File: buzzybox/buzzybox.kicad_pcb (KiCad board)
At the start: 2 copper layers, 116.8 x 71.1 mm, 67 parts, among them J1 AudioJack2, J2 Barrel_Jack, Q1 Q_NPN_EBC, Q10 Q_NPN_EBC, Q2 Q_NPN_EBC, Q3 Q_NPN_EBC, Q4 Q_NPN_EBC, Q5 Q_NPN_EBC, Q6 Q_NPN_EBC, Q7 Q_NPN_EBC, Q8 Q_NPN_EBC, Q9 Q_NPN_EBC

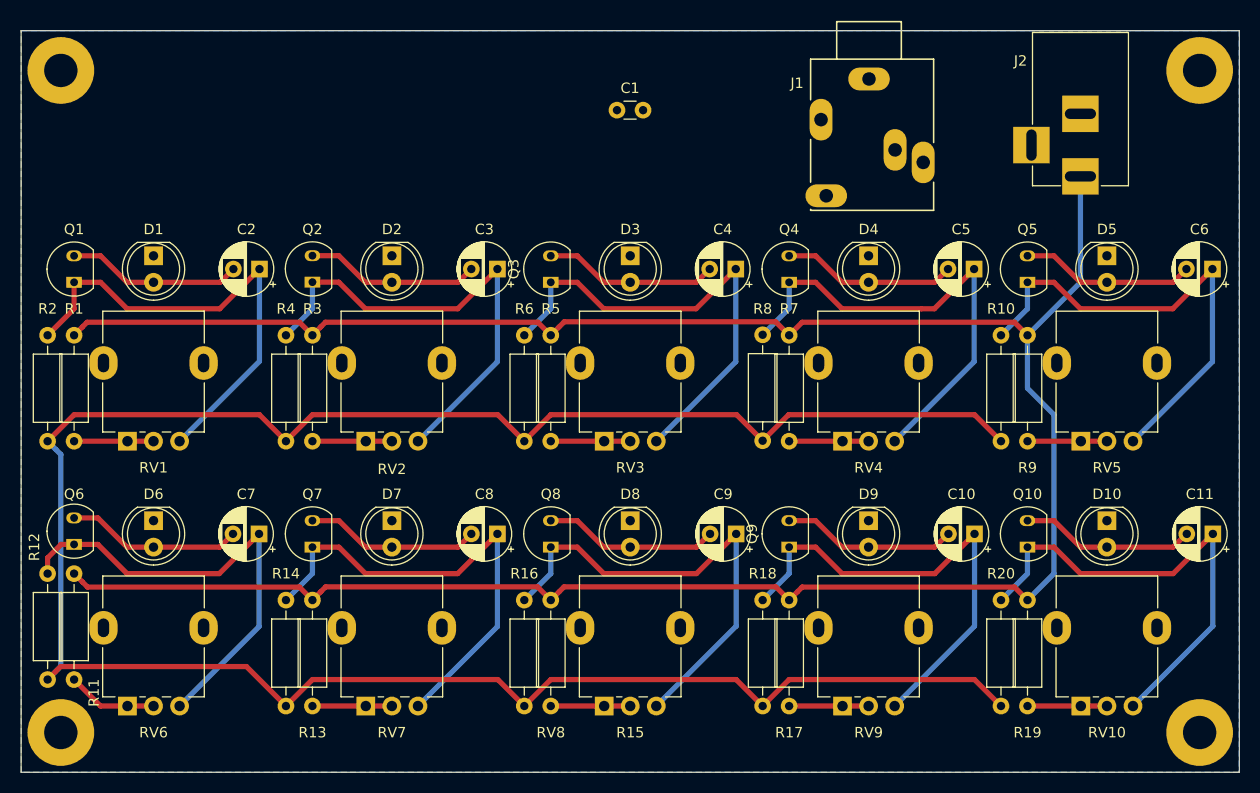
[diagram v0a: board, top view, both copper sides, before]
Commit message: complete mini layout
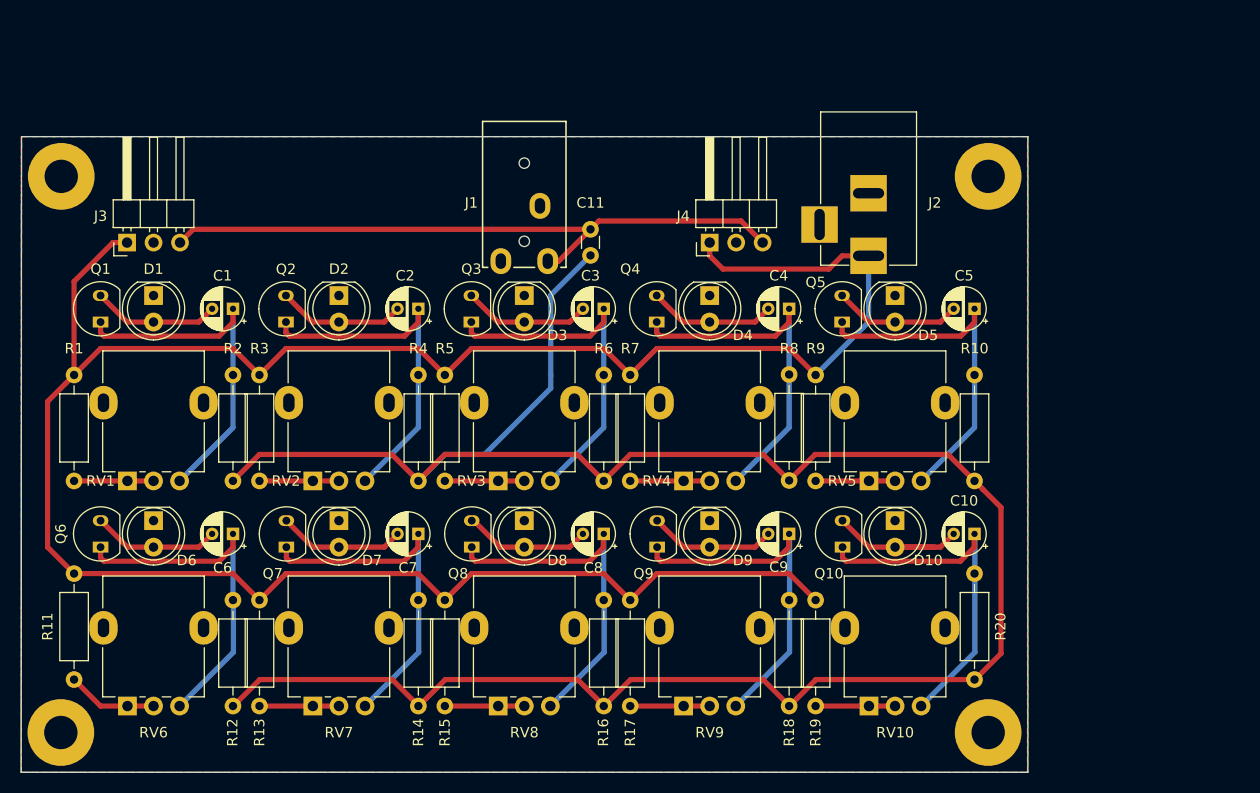
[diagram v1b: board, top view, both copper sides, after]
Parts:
- removed the C11 at (177.8, 87.6)
- added C1: CP1, Capacitor_THT:CP_Radial_D4.0mm_P2.00mm, F.Cu at (83.8, 66.0)
- added J3: Conn_01x03, Connector_PinHeader_2.54mm:PinHeader_1x03_P2.54mm_Horizontal, F.Cu at (73.7, 59.7)
- added J4: Conn_01x03, Connector_PinHeader_2.54mm:PinHeader_1x03_P2.54mm_Horizontal, F.Cu at (129.5, 59.7)
- C10, C2, C3, C4, C5, C6, C7, C8, C9: value C -> CP1; footprint Capacitor_THT:CP_Radial_D5.0mm_P2.50mm -> Capacitor_THT:CP_Radial_D4.0mm_P2.00mm
- J1: value AudioJack2 -> AudioJack3; footprint Connectors:Stereo_Jack_3.5mm_Switch_Ledino_KB3SPRS -> buzzybox:STX-3000
- Q1, Q10, Q2, Q3, Q4, Q5, Q6, Q7, Q8, Q9: value Q_NPN_EBC -> NPN
- moved C6 97.3 mm to (83.8, 87.6)
- moved J1 28.8 mm to (111.8, 52.1), turned to 0 degrees
- moved H2 22.7 mm to (156.2, 53.3)
- moved J2 21.7 mm to (144.8, 61.0)
- moved R9 20.7 mm to (139.7, 72.4)
- moved D5 20.7 mm to (147.3, 64.8)
- moved RV5 20.7 mm to (144.8, 82.5)
- moved R19 20.3 mm to (139.7, 94.0)
- moved D10 20.3 mm to (147.3, 86.4)
- moved RV10 20.3 mm to (144.8, 104.1)
- moved H3 20.3 mm to (156.2, 106.7)
- moved Q5 18.2 mm to (142.2, 67.3)
- moved R2 18.2 mm to (83.8, 82.5)
- moved R12 18.0 mm to (83.8, 104.1)
- moved Q10 17.7 mm to (142.3, 88.9)
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- renumbered C1 to C11
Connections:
- C11 pad 2: Net-(C1-Pad2) -> Net-(C11-Pad2)
- D1 pad 2: Net-(C2-Pad2) -> Net-(C1-Pad2)
- D10 pad 2: Net-(C11-Pad2) -> Net-(C10-Pad2)
- D2 pad 2: Net-(C3-Pad2) -> Net-(C2-Pad2)
- D3 pad 2: Net-(C4-Pad2) -> Net-(C3-Pad2)
- D4 pad 2: Net-(C5-Pad2) -> Net-(C4-Pad2)
- D5 pad 2: Net-(C6-Pad2) -> Net-(C5-Pad2)
- D6 pad 2: Net-(C7-Pad2) -> Net-(C6-Pad2)
- D7 pad 2: Net-(C8-Pad2) -> Net-(C7-Pad2)
- D8 pad 2: Net-(C9-Pad2) -> Net-(C8-Pad2)
- D9 pad 2: Net-(C10-Pad2) -> Net-(C9-Pad2)
- Q1 pad 1: Net-(C2-Pad1) -> Net-(C1-Pad1)
- Q1 pad 3: Net-(C2-Pad2) -> Net-(C1-Pad2)
- Q10 pad 1: Net-(C11-Pad1) -> Net-(C10-Pad1)
- Q10 pad 3: Net-(C11-Pad2) -> Net-(C10-Pad2)
- Q2 pad 1: Net-(C3-Pad1) -> Net-(C2-Pad1)
- Q2 pad 3: Net-(C3-Pad2) -> Net-(C2-Pad2)
- Q3 pad 1: Net-(C4-Pad1) -> Net-(C3-Pad1)
- Q3 pad 3: Net-(C4-Pad2) -> Net-(C3-Pad2)
- Q4 pad 1: Net-(C5-Pad1) -> Net-(C4-Pad1)
- Q4 pad 3: Net-(C5-Pad2) -> Net-(C4-Pad2)
- Q5 pad 1: Net-(C6-Pad1) -> Net-(C5-Pad1)
- Q5 pad 3: Net-(C6-Pad2) -> Net-(C5-Pad2)
- Q6 pad 1: Net-(C7-Pad1) -> Net-(C6-Pad1)
- Q6 pad 3: Net-(C7-Pad2) -> Net-(C6-Pad2)
- Q7 pad 1: Net-(C8-Pad1) -> Net-(C7-Pad1)
- Q7 pad 3: Net-(C8-Pad2) -> Net-(C7-Pad2)
- Q8 pad 1: Net-(C9-Pad1) -> Net-(C8-Pad1)
- Q8 pad 3: Net-(C9-Pad2) -> Net-(C8-Pad2)
- Q9 pad 1: Net-(C10-Pad1) -> Net-(C9-Pad1)
- Q9 pad 3: Net-(C10-Pad2) -> Net-(C9-Pad2)
- R10 pad 2: Net-(C6-Pad1) -> Net-(C5-Pad1)
- R12 pad 2: Net-(C7-Pad1) -> Net-(C6-Pad1)
- R14 pad 2: Net-(C8-Pad1) -> Net-(C7-Pad1)
- R16 pad 2: Net-(C9-Pad1) -> Net-(C8-Pad1)
- R18 pad 2: Net-(C10-Pad1) -> Net-(C9-Pad1)
- R2 pad 2: Net-(C2-Pad1) -> Net-(C1-Pad1)
- R20 pad 2: Net-(C11-Pad1) -> Net-(C10-Pad1)
- R4 pad 2: Net-(C3-Pad1) -> Net-(C2-Pad1)
- R6 pad 2: Net-(C4-Pad1) -> Net-(C3-Pad1)
- R8 pad 2: Net-(C5-Pad1) -> Net-(C4-Pad1)
- RV1 pad 3: Net-(C2-Pad1) -> Net-(C1-Pad1)
- RV10 pad 3: Net-(C11-Pad1) -> Net-(C10-Pad1)
- RV2 pad 3: Net-(C3-Pad1) -> Net-(C2-Pad1)
- RV3 pad 3: Net-(C4-Pad1) -> Net-(C3-Pad1)
- RV4 pad 3: Net-(C5-Pad1) -> Net-(C4-Pad1)
- RV5 pad 3: Net-(C6-Pad1) -> Net-(C5-Pad1)
- RV6 pad 3: Net-(C7-Pad1) -> Net-(C6-Pad1)
- RV7 pad 3: Net-(C8-Pad1) -> Net-(C7-Pad1)
- RV8 pad 3: Net-(C9-Pad1) -> Net-(C8-Pad1)
- RV9 pad 3: Net-(C10-Pad1) -> Net-(C9-Pad1)
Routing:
- net Net-(C11-Pad1): track 46.2 -> 0.00 mm
- net Net-(C11-Pad2): track 16.8 -> 63.0 mm
- net Net-(C1-Pad1): track 0.00 -> 34.3 mm
- net /oscillator/OSC_OUT: track 223.6 -> 209.8 mm
- net Net-(C1-Pad2): track 0.00 -> 12.3 mm
- net Net-(C9-Pad1): track 46.2 -> 34.3 mm
- net Net-(C10-Pad1): track 46.2 -> 34.3 mm
- net Net-(C8-Pad1): track 46.2 -> 34.3 mm
- net Net-(C2-Pad1): track 46.2 -> 34.3 mm
- net Net-(C3-Pad1): track 46.2 -> 34.3 mm
- net Net-(C4-Pad1): track 46.2 -> 34.3 mm
- net Net-(C6-Pad1): track 46.2 -> 34.4 mm
- net Net-(C5-Pad1): track 46.1 -> 34.3 mm
- net Net-(C7-Pad1): track 44.7 -> 34.3 mm
- net +VDC: track 235.2 -> 225.9 mm
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- added copper zone on F.Cu, net -VDC
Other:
- board size 116.8 x 71.1 mm -> 96.6 x 61 mm
- board text added: "+VDC GND AUD"
- board text added: "JLCJLCJLCJLC"
